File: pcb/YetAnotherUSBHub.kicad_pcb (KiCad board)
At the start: 2 copper layers, 77.6 x 32.6 mm, 24 parts, among them J1 USB_A, J2 USB_A, J3 Micro_SD_Card, J4 USB_C_Receptacle_USB2.0_14P, J5 USB_C_Receptacle_USB2.0_14P, U2 GL823K-HCY04

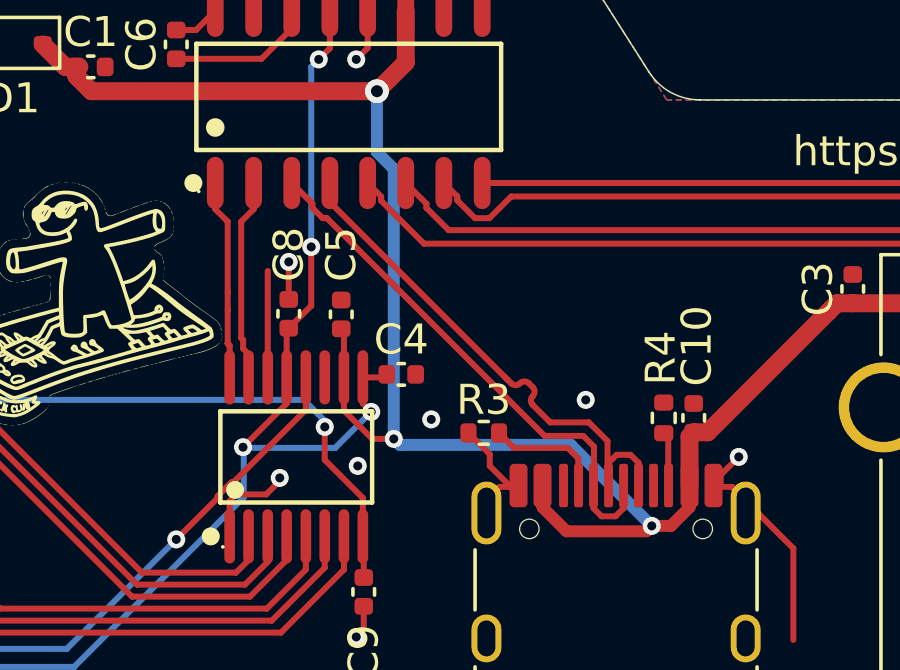
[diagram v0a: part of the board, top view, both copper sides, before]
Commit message: stuff
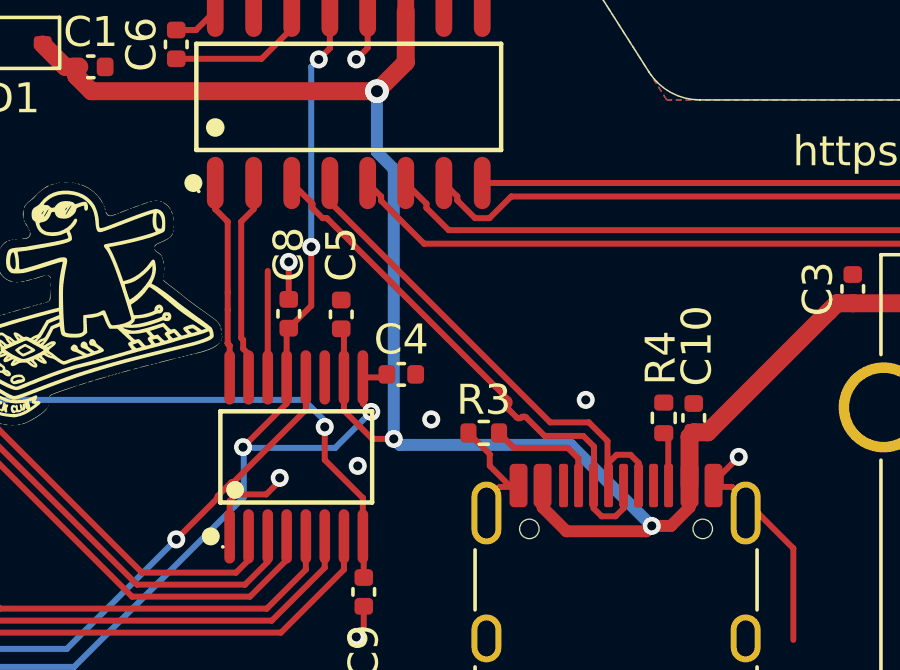
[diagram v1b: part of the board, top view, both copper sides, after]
